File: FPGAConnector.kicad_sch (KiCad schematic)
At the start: 1 part

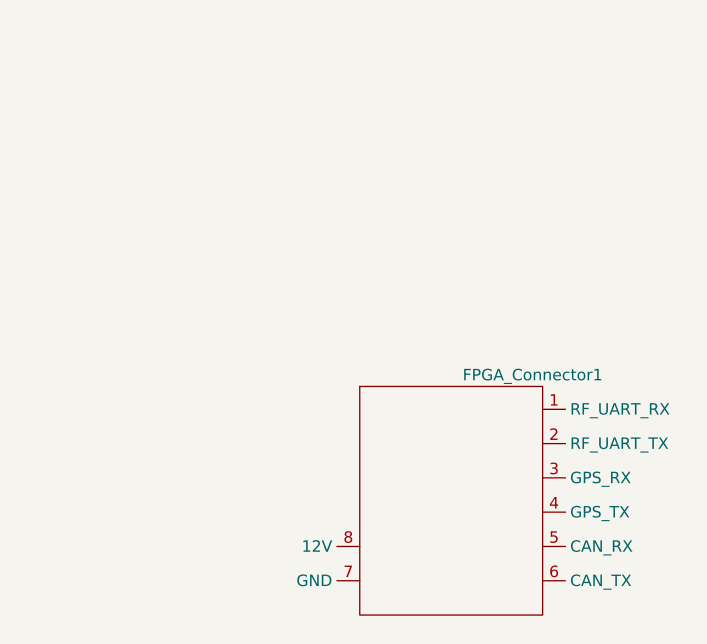
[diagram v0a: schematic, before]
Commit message: power/connectors
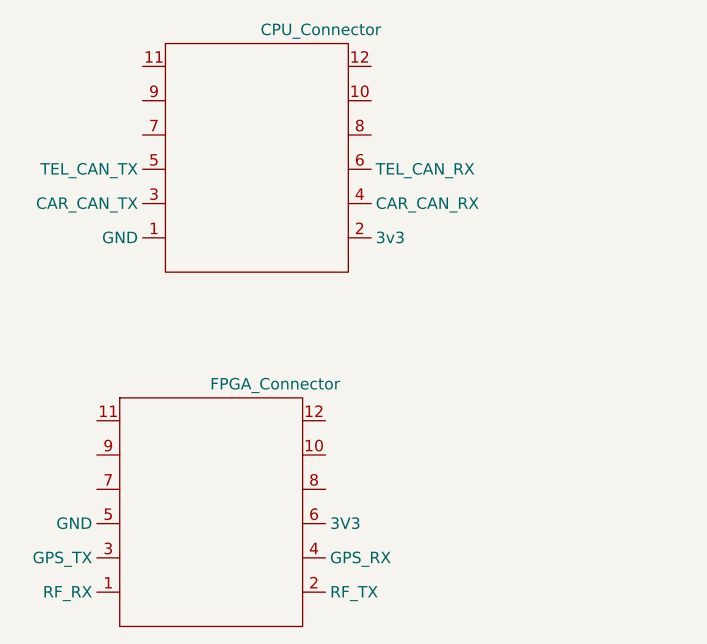
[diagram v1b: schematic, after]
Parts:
- removed FPGA_Connector1: ~, symbol FPGA_Connector:FPGA_Connector
- added CPU_Connector, FPGA_Connector: ~, symbol FPGA_Connector:FPGA_Connector
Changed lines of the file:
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@@
 	(paper "A4")
 	(symbol
+		(lib_name "FPGA_Connector_1")
 		(lib_id "FPGA_Connector:FPGA_Connector")
-		(at 146.05 93.98 0)
+		(at 124.46 55.88 0)
 		(unit 1)
 		(exclude_from_sim no)
@@
 		(on_board yes)
 		(dnp no)
-		(fields_autoplaced yes)
-		(property "Reference" "FPGA_Connector1"
-			(at 147.32 80.01 0)
+		(property "Reference" "CPU_Connector"
+			(at 131.572 41.656 0)
 			(effects
 				(font
 					(size 1.27 1.27)
 				)
-				(justify left)
 			)
 		)
 		(property "Value" "~"
-			(at 160.02 95.2499 0)
+			(at 124.46 40.64 0)
 			(effects
 				(font
 					(size 1.27 1.27)
 				)
-				(justify left)
 			)
 		)
 		(property "Footprint" ""
-			(at 146.05 93.98 0)
+			(at 124.46 55.88 0)
 			(effects
 				(font
@@
 		)
 		(property "Datasheet" ""
-			(at 146.05 93.98 0)
+			(at 124.46 55.88 0)
 			(effects
 				(font
@@
 		)
 		(property "Description" ""
-			(at 146.05 93.98 0)
+			(at 124.46 55.88 0)
 			(effects
 				(font
@@
 			)
 		)
-		(pin "7"
+		(pin "3"
 		)
 		(pin "1"
@@
 		(pin "4"
 		)
-		(pin "3"
+		(pin "8"
 		)
 		(pin "5"
 		)
-		(pin "8"
+		(pin "11"
 		)
 		(pin "6"
 		)
+		(pin "7"
+		)
+		(pin "12"
+		)
+		(pin "9"
+		)
+		(pin "10"
+		)
 		(instances
-			(project ""
+			(project "TSOMProject"
 				(path "/f13eb969-5de0-437e-a1b7-e0204111e0b2/555dcf2f-9cf7-4916-9b4f-3a8f620095c0"
-					(reference "FPGA_Connector1")
+					(reference "CPU_Connector")
 					(unit 1)
 				)
-				(path "/f13eb969-5de0-437e-a1b7-e0204111e0b2/5da8fdf4-ad8c-47df-b08e-df168b9b0cb6"
-					(reference "FPGA_Connector1")
+			)
+		)
+	)
+	(symbol
+		(lib_name "FPGA_Connector_2")
+		(lib_id "FPGA_Connector:FPGA_Connector")
+		(at 119.38 95.25 0)
+		(unit 1)
+		(exclude_from_sim no)
+		(in_bom yes)
+		(on_board yes)
+		(dnp no)
+		(property "Reference" "FPGA_Connector"
+			(at 126.492 81.026 0)
+			(effects
+				(font
+					(size 1.27 1.27)
+				)
+			)
+		)
+		(property "Value" "~"
+			(at 119.38 80.01 0)
+			(effects
+				(font
+					(size 1.27 1.27)
+				)
+			)
+		)
+		(property "Footprint" ""
+			(at 119.38 95.25 0)
+			(effects
+				(font
+					(size 1.27 1.27)
+				)
+				(hide yes)
+			)
+		)
+		(property "Datasheet" ""
+			(at 119.38 95.25 0)
+			(effects
+				(font
+					(size 1.27 1.27)
+				)
+				(hide yes)
+			)
+		)
+		(property "Description" ""
+			(at 119.38 95.25 0)
+			(effects
+				(font
+					(size 1.27 1.27)
+				)
+				(hide yes)
+			)
+		)
+		(pin "3"
+		)
+		(pin "1"
+		)
+		(pin "2"
+		)
+		(pin "4"
+		)
+		(pin "8"
+		)
+		(pin "5"
+		)
+		(pin "11"
+		)
+		(pin "6"
+		)
+		(pin "7"
+		)
+		(pin "12"
+		)
+		(pin "9"
+		)
+		(pin "10"
+		)
+		(instances
+			(project "TSOMProject"
+				(path "/f13eb969-5de0-437e-a1b7-e0204111e0b2/555dcf2f-9cf7-4916-9b4f-3a8f620095c0"
+					(reference "FPGA_Connector")
 					(unit 1)
 				)

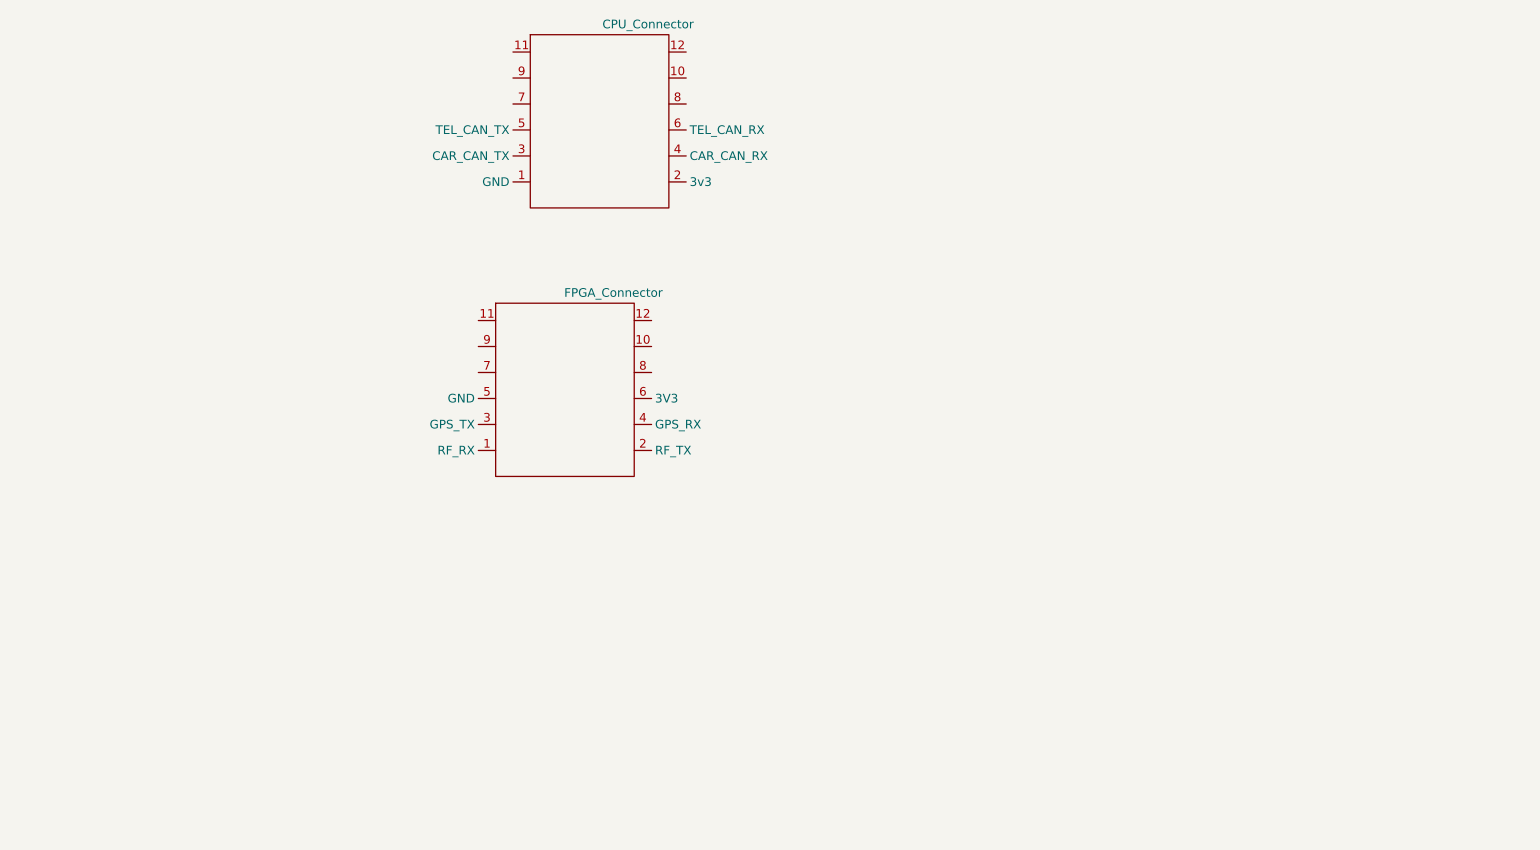
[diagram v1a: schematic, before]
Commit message: fix errors schem
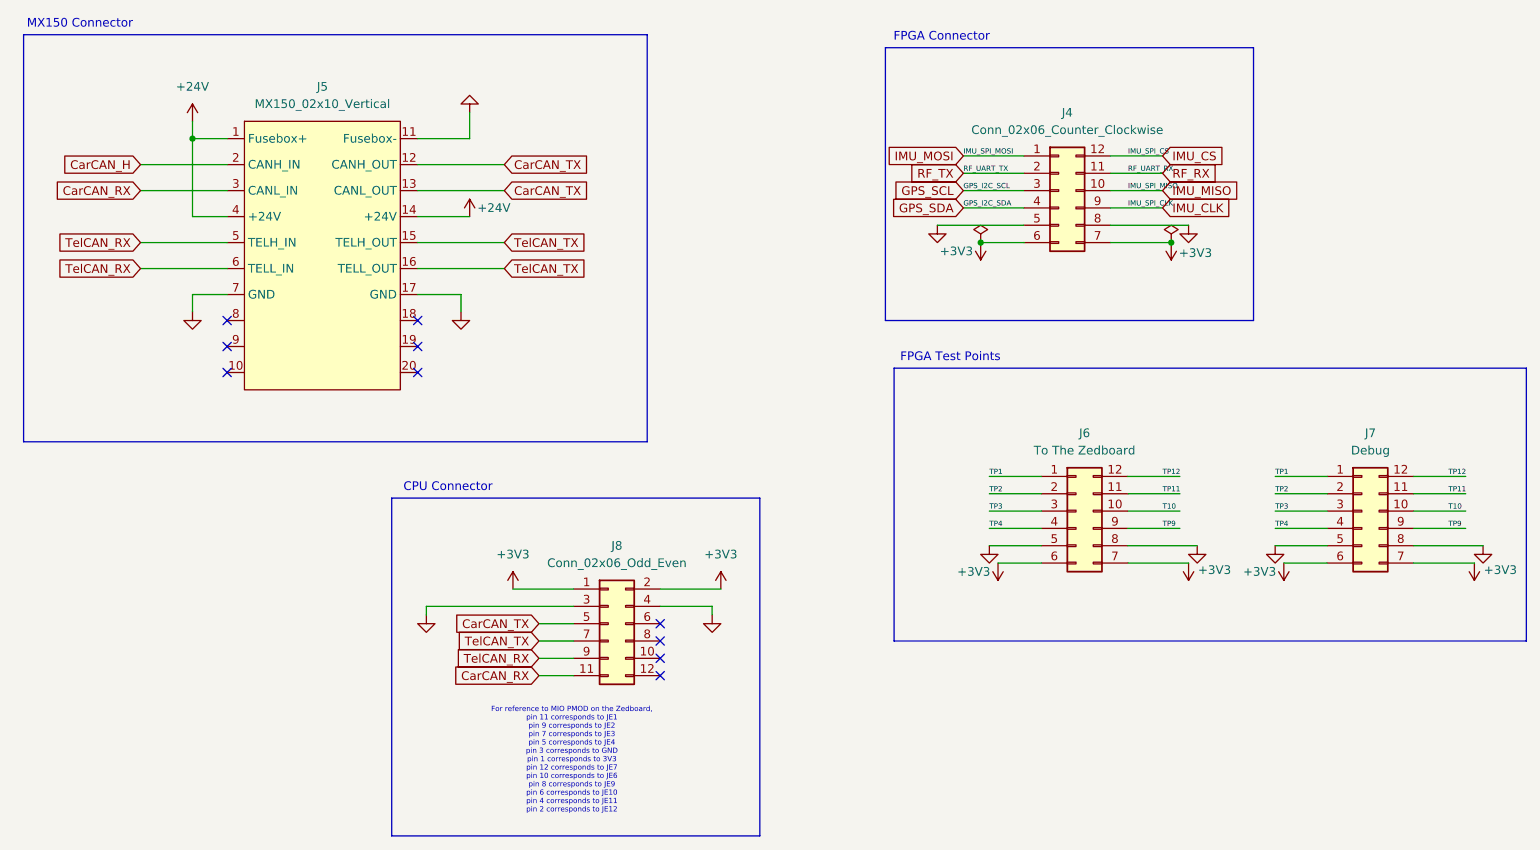
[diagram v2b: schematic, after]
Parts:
- removed CPU_Connector, FPGA_Connector: ~, symbol FPGA_Connector:FPGA_Connector
- added J4: Conn_02x06_Counter_Clockwise, symbol Connector_Generic:Conn_02x06_Counter_Clockwise
- added J5: MX150_02x10_Vertical, UTSVT_Connectors:MX150_02x10_Vertical, symbol utsvt_connectors:MX150_02x10_Vertical
- added J6: To The Zedboard, symbol Connector_Generic:Conn_02x06_Counter_Clockwise
- added J7: Debug, symbol Connector_Generic:Conn_02x06_Counter_Clockwise
- added J8: Conn_02x06_Odd_Even, symbol Connector_Generic:Conn_02x06_Odd_Even
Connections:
- new net +24V: J5.1 (Fusebox+), J5.14 (+24V), J5.4 (+24V)
- new net +3V3: J4.6 (Pin_6), J4.7 (Pin_7), J6.6 (Pin_6), J6.7 (Pin_7), J7.6 (Pin_6), J7.7 (Pin_7), J8.1 (Pin_1), J8.2 (Pin_2)
- new net CarCAN_H: J5.2 (CANH_IN)
- new net CarCAN_RX: J5.3 (CANL_IN), J8.11 (Pin_11)
- new net CarCAN_TX: J5.12 (CANH_OUT), J5.13 (CANL_OUT), J8.5 (Pin_5)
- new net GND: J4.5 (Pin_5), J4.8 (Pin_8), J5.11 (Fusebox-), J5.17 (GND), J5.7 (GND), J6.5 (Pin_5), J6.8 (Pin_8), J7.5 (Pin_5), J7.8 (Pin_8), J8.3 (Pin_3), J8.4 (Pin_4)
- new net GPS_SCL: J4.3 (Pin_3)
- new net GPS_SDA: J4.4 (Pin_4)
- new net IMU_CLK: J4.9 (Pin_9)
- new net IMU_CS: J4.12 (Pin_12)
- new net IMU_MISO: J4.10 (Pin_10)
- new net IMU_MOSI: J4.1 (Pin_1)
- new net RF_RX: J4.11 (Pin_11)
- new net RF_TX: J4.2 (Pin_2)
- new net T10: J6.10 (Pin_10), J7.10 (Pin_10)
- new net TP1: J6.1 (Pin_1), J7.1 (Pin_1)
- new net TP11: J6.11 (Pin_11), J7.11 (Pin_11)
- new net TP12: J6.12 (Pin_12), J7.12 (Pin_12)
- new net TP2: J6.2 (Pin_2), J7.2 (Pin_2)
- new net TP3: J6.3 (Pin_3), J7.3 (Pin_3)
- new net TP4: J6.4 (Pin_4), J7.4 (Pin_4)
- new net TP9: J6.9 (Pin_9), J7.9 (Pin_9)
- new net TelCAN_RX: J5.5 (TELH_IN), J5.6 (TELL_IN), J8.9 (Pin_9)
- new net TelCAN_TX: J5.15 (TELH_OUT), J5.16 (TELL_OUT), J8.7 (Pin_7)
- no-connect marks 0 -> 10
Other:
- note added: "CPU Connector"
- note added: "FPGA Connector"
- note added: "FPGA Test Points"
- note added: "For reference to MIO PMOD on the Zedboard, pin 11 corresponds to JE1 pin 9 corresponds to JE2 pin 7 corresponds to JE3 pin 5 corresponds to JE4 pin 3 corresponds to GND pin 1 corresponds to 3V3 pin 12 corresponds to JE7 pin 10 corresponds to JE6 pin 8 corresponds to JE9 pin 6 corresponds to JE10 pin 4 corresponds to JE11 pin 2 corresponds to JE12"
- note added: "MX150 Connector"
